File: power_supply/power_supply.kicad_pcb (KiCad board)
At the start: 2 copper layers, 100 x 100 mm, 36 parts, among them J1 Conn_01x02_Socket, J10 Conn_01x02_Socket, J11 Conn_01x02_Socket, J12 Conn_01x02_Socket, J13 Conn_01x02_Socket, J14 Conn_01x02_Socket, J15 Conn_01x02_Socket, J16 Conn_01x02_Socket, J17 Conn_01x02_Socket, J18 Conn_01x02_Socket, J19 Conn_01x02_Socket, J2 Conn_01x02_Socket, J20 Conn_01x02_Socket, J21 Conn_01x02_Pin, J22 Conn_01x02_Pin, J23 Conn_01x02_Socket, J24 Conn_01x02_Socket, J3 Conn_01x02_Socket, J4 Conn_01x02_Socket, J5 Conn_01x02_Socket, J6 Conn_01x02_Socket, J7 Conn_01x02_Socket, J8 Conn_01x02_Socket, J9 Conn_01x02_Socket

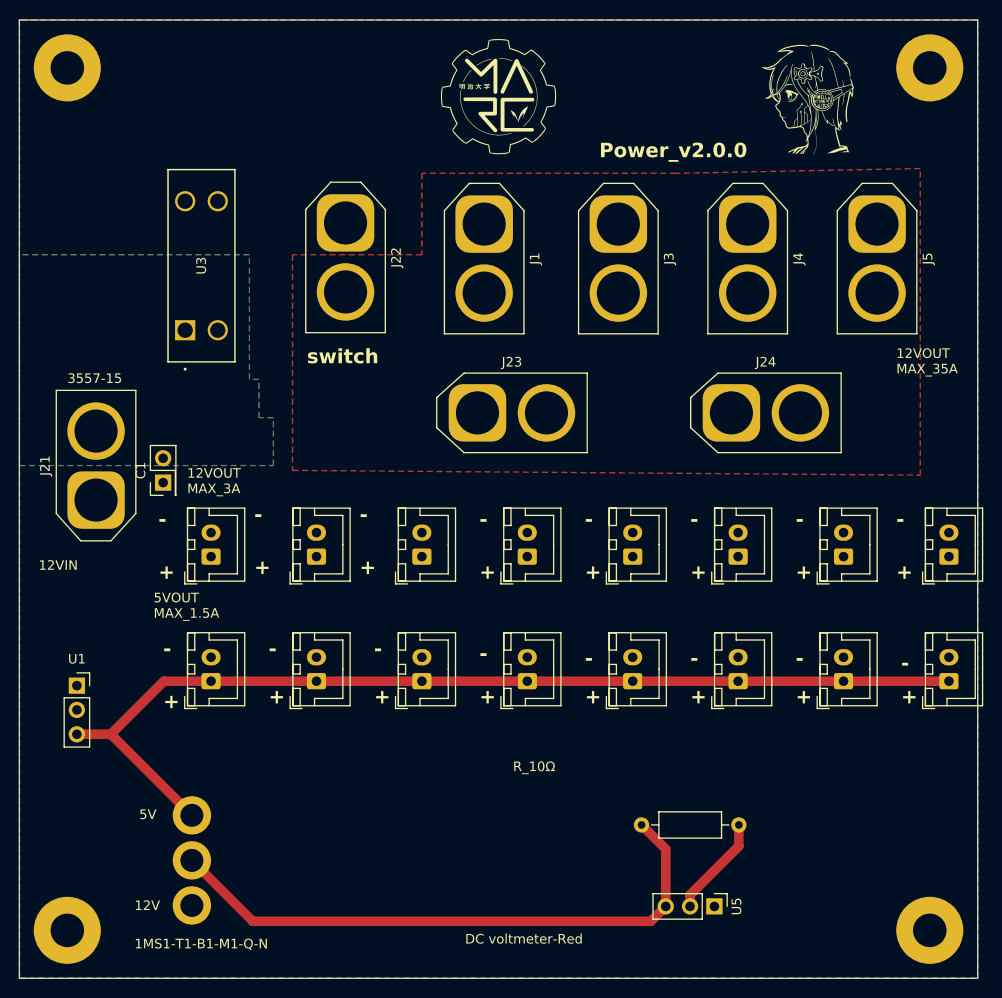
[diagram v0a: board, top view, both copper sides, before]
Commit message: 2024/11/08
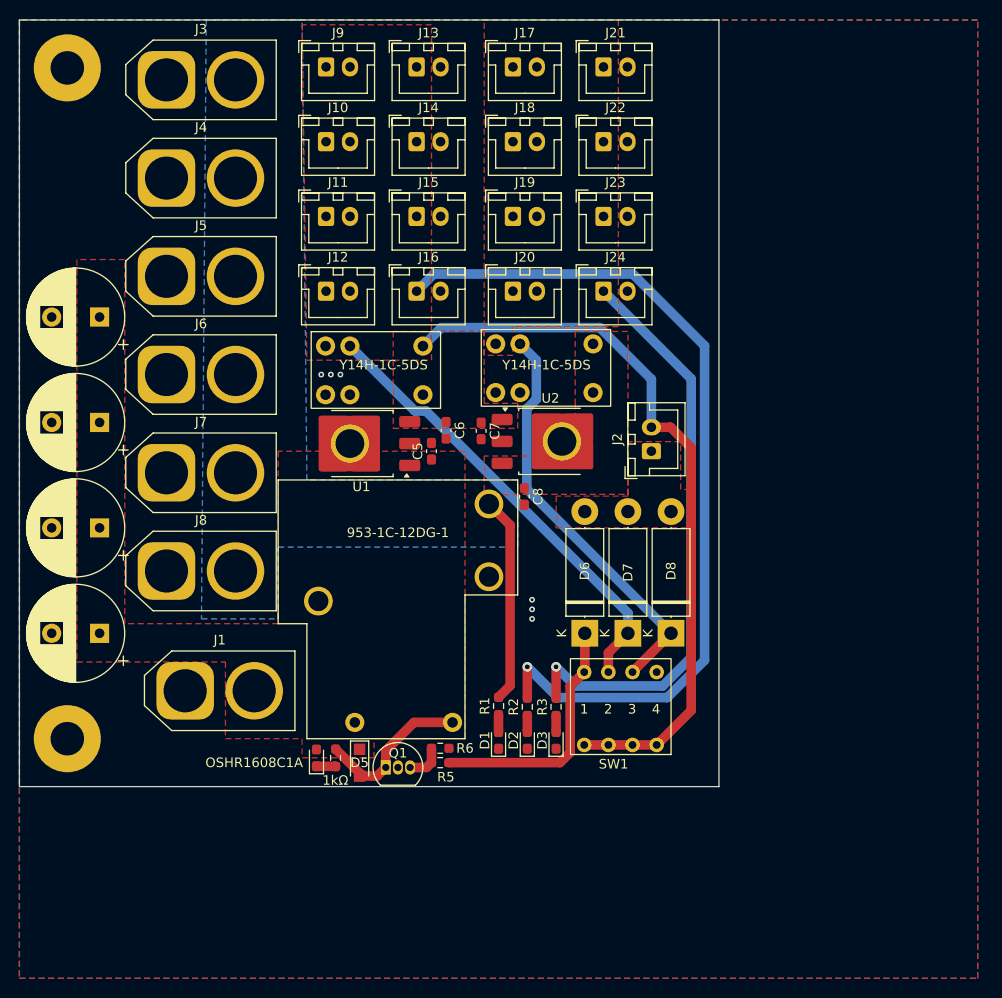
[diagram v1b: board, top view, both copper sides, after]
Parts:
- removed the G*** at (62.0, 20.0)
- removed the REF** at (107.0, 17.0)
- removed the REF** at (107.0, 107.0)
- added C2: C_Polarized, Capacitor_THT:CP_Radial_D10.0mm_P5.00mm, F.Cu at (20.4, 54.0)
- added C3: C_Polarized, Capacitor_THT:CP_Radial_D10.0mm_P5.00mm, F.Cu at (20.4, 65.0)
- added C4: C_Polarized, Capacitor_THT:CP_Radial_D10.0mm_P5.00mm, F.Cu at (20.4, 76.0)
- added C5: 0.33μF, Capacitor_SMD:C_0603_1608Metric_Pad1.08x0.95mm_HandSolder, F.Cu at (55.0, 57.0)
- added C6: 0.1μF, Capacitor_SMD:C_0603_1608Metric_Pad1.08x0.95mm_HandSolder, F.Cu at (56.5, 54.8)
- added C7: 0.33μF, Capacitor_SMD:C_0603_1608Metric_Pad1.08x0.95mm_HandSolder, F.Cu at (60.2, 54.9)
- added C8: 0.1μF, Capacitor_SMD:C_0603_1608Metric_Pad1.08x0.95mm_HandSolder, F.Cu at (64.7, 61.7)
- added D1: LED, LED_SMD:LED_0603_1608Metric_Pad1.05x0.95mm_HandSolder, F.Cu at (62.0, 87.2)
- added D2: LED, LED_SMD:LED_0603_1608Metric_Pad1.05x0.95mm_HandSolder, F.Cu at (65.0, 87.2)
- added D3: LED, LED_SMD:LED_0603_1608Metric_Pad1.05x0.95mm_HandSolder, F.Cu at (68.0, 87.2)
- added D4: OSHR1608C1A, LED_SMD:LED_0603_1608Metric_Pad1.05x0.95mm_HandSolder, F.Cu at (43.0, 89.0)
- added D5: GS1010FL, Diode_SMD:Nexperia_CFP3_SOD-123W, F.Cu at (47.5, 89.5)
- added D6: D, Diode_THT:D_5W_P12.70mm_Horizontal, F.Cu at (71.0, 76.0)
- added D7: D, Diode_THT:D_5W_P12.70mm_Horizontal, F.Cu at (75.5, 76.0)
- added D8: D, Diode_THT:D_5W_P12.70mm_Horizontal, F.Cu at (80.0, 76.0)
- added Q1: 2SC945L-K-T92-K, Package_TO_SOT_THT:TO-92_Inline, F.Cu at (50.2, 90.0)
- added R2: 300Ω, Resistor_SMD:R_0603_1608Metric_Pad0.98x0.95mm_HandSolder, F.Cu at (65.0, 83.7)
- added R3: 120Ω, Resistor_SMD:R_0603_1608Metric_Pad0.98x0.95mm_HandSolder, F.Cu at (68.0, 83.7)
- added R4: 1kΩ, Resistor_SMD:R_0603_1608Metric_Pad0.98x0.95mm_HandSolder, F.Cu at (45.0, 89.0)
- added R5: 1kΩ, Resistor_SMD:R_0603_1608Metric_Pad0.98x0.95mm_HandSolder, F.Cu at (55.9, 89.5)
- added R6: 10kΩ, Resistor_SMD:R_0603_1608Metric_Pad0.98x0.95mm_HandSolder, F.Cu at (55.9, 88.0)
- added SW1: SW_DIP_x04, 00a:KSD42, F.Cu at (78.5, 87.7)
- added U2: NJM2845DL1-33, 00a:TO-252-3_TabPin2, F.Cu at (67.4, 56.0)
- C1: value C -> C_Polarized; footprint Connector_PinHeader_2.54mm:PinHeader_2x01_P2.54mm_Vertical -> Capacitor_THT:CP_Radial_D10.0mm_P5.00mm
- G***: moved to B.Cu
- J1: value Conn_01x02_Socket -> XT60_IN
- J10, J11, J12, J13, J14, J15, J16, J9: value Conn_01x02_Socket -> XH_OUT
- J17, J18, J19, J20: value Conn_01x02_Socket -> XH_3.3V_OUT
- J2: value Conn_01x02_Socket -> Emergency Stop Switch
- J21, J22: value Conn_01x02_Pin -> XH_3.3V_OUT; footprint Connector_AMASS:AMASS_XT60-F_1x02_P7.20mm_Vertical -> Connector_JST:JST_XH_B2B-XH-A_1x02_P2.50mm_Vertical
- J23, J24: value Conn_01x02_Socket -> XH_3.3V_OUT; footprint Connector_AMASS:AMASS_XT60-F_1x02_P7.20mm_Vertical -> Connector_JST:JST_XH_B2B-XH-A_1x02_P2.50mm_Vertical
- J3, J4, J5: value Conn_01x02_Socket -> XT60_OUT
- J6, J7, J8: value Conn_01x02_Socket -> XT60_OUT; footprint Connector_JST:JST_XH_B2B-XH-A_1x02_P2.50mm_Vertical -> Connector_AMASS:AMASS_XT60-F_1x02_P7.20mm_Vertical
- R1: value 10 -> 1kΩ; footprint Resistor_THT:R_Axial_DIN0207_L6.3mm_D2.5mm_P10.16mm_Horizontal -> Resistor_SMD:R_0603_1608Metric_Pad0.98x0.95mm_HandSolder
- U1: value ~ -> NJM7805SDL1; footprint Connector_PinSocket_2.54mm:PinSocket_1x03_P2.54mm_Vertical -> 00a:TO-252-3_TabPin2
- U3: value ~ -> 953-1C-12DG-1; footprint footprints:3557-15_KEY -> 00a:953-1C-12DG-1
- U4: value ~ -> Y14H-1C-5DS; footprint 00a:1MS1-T1-B1-M1-Q-N-S -> 00a:Y14H-1C-5DS
- U5: value ~ -> Y14H-1C-5DS; footprint Connector_PinHeader_2.54mm:PinHeader_1x03_P2.54mm_Vertical -> 00a:Y14H-1C-5DS
- moved J13 75.5 mm to (53.5, 16.9), turned to 0 degrees
- moved J5 74.4 mm to (27.4, 38.8), turned to 0 degrees
- moved G*** 72.5 mm to (64.3, 85.7), turned to 180 degrees
- moved J21 69.6 mm to (73.0, 16.9), turned to 0 degrees
- moved J17 65.3 mm to (63.5, 16.9), turned to 0 degrees
- moved U5 63.0 mm to (61.7, 45.8), turned to 0 degrees
- moved J20 61.0 mm to (63.5, 40.3), turned to 0 degrees
- moved J18 61.0 mm to (63.5, 24.7), turned to 0 degrees
- moved J4 60.8 mm to (27.4, 28.5), turned to 0 degrees
- moved J12 60.7 mm to (44.0, 40.3), turned to 0 degrees
- moved J19 59.5 mm to (63.5, 32.5), turned to 0 degrees
- moved J1 57.8 mm to (29.3, 82.0), turned to 0 degrees
- moved J14 57.3 mm to (53.5, 24.7), turned to 0 degrees
- moved J11 55.8 mm to (44.0, 32.5), turned to 0 degrees
- moved J9 55.2 mm to (44.0, 16.9), turned to 0 degrees
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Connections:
- C1 pad 1: GND -> +12V_IN
- C1 pad 2: +12V_1 -> GND
- J1 pad 2: +12V_3 -> +12V_IN
- J10 pad 1: +12V_2 -> +5V_OUT
- J11 pad 1: +12V_2 -> +5V_OUT
- J12 pad 1: +12V_2 -> +5V_OUT
- J13 pad 1: +12V_2 -> +5V_OUT
- J14 pad 1: Net-(J14-Pin_1) -> +5V_OUT
- J15 pad 1: Net-(J14-Pin_1) -> +5V_OUT
- J16 pad 1: Net-(J14-Pin_1) -> +5V_OUT
- J17 pad 1: Net-(J14-Pin_1) -> +3.3V_OUT
- J18 pad 1: Net-(J14-Pin_1) -> +3.3V_OUT
- J19 pad 1: Net-(J14-Pin_1) -> +3.3V_OUT
- J2 pad 1: Net-(J14-Pin_1) -> Net-(D6-A)
- J2 pad 2: GND -> +5V_IN
- J20 pad 1: Net-(J14-Pin_1) -> +3.3V_OUT
- J21 pad 1: GND -> +3.3V_OUT
- J21 pad 2: +12V_1 -> GND
- J22 pad 1: +12V_2 -> +3.3V_OUT
- J22 pad 2: +12V_3 -> GND
- J23 pad 1: GND -> +3.3V_OUT
- J23 pad 2: +12V_3 -> GND
- J24 pad 1: GND -> +3.3V_OUT
- J24 pad 2: +12V_3 -> GND
- J3 pad 2: +12V_3 -> +12V_OUT
- J4 pad 2: +12V_3 -> +12V_OUT
- J5 pad 2: +12V_3 -> +12V_OUT
- J6 pad 1: +12V_2 -> GND
- J6 pad 2: GND -> +12V_OUT
- J7 pad 1: +12V_2 -> GND
- J7 pad 2: GND -> +12V_OUT
- J8 pad 1: +12V_2 -> GND
- J8 pad 2: GND -> +12V_OUT
- J9 pad 1: +12V_2 -> +5V_OUT
- R1 pad 1: Net-(R1-Pad1) -> Net-(D1-A)
- R1 pad 2: Net-(U5-OUT) -> +12V_OUT
- U1 pad 1: +12V_2 -> +12V_IN
- U1 pad 3: Net-(J14-Pin_1) -> +5V_IN
- U3 pad 1: +12V_1 -> +12V_IN
- U3 pad 2: +12V_1 -> Net-(D5-A)
- U3 pad 3: +12V_2 -> +12_IN
- U3 pad 4: +12V_2 -> unconnected-(U3-N.O.-Pad4)
- U4 pad 1: Net-(J14-Pin_1) -> +5V_OUT
- U4 pad 2: Net-(U5-OUT) -> unconnected-(U4-N.O.-Pad2)
- U4 pad 3: +12V_2 -> Net-(D7-K)
- U5 pad 1: GND -> +3.3V_OUT
- U5 pad 2: Net-(R1-Pad1) -> unconnected-(U5-N.O.-Pad2)
- U5 pad 3: Net-(U5-OUT) -> Net-(D8-K)
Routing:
- net Net-(J14-Pin_1): track 105.3 -> 0.00 mm
- net +5V_OUT: track 0.00 -> 91.4 mm, vias 0 -> 1
- net +5V_IN: track 0.00 -> 77.0 mm
- net Net-(U5-OUT): track 62.3 -> 0.00 mm
- net +3.3V_OUT: track 0.00 -> 61.4 mm, vias 0 -> 1
- net Net-(D7-K): track 0.00 -> 47.6 mm
- net Net-(D8-K): track 0.00 -> 43.3 mm
- net Net-(D6-K): track 0.00 -> 26.2 mm
- net +12V_OUT: track 0.00 -> 21.6 mm
- net Net-(D5-A): track 0.00 -> 16.9 mm
- net Net-(R1-Pad1): track 10.6 -> 0.00 mm
- net Net-(Q1-B): track 0.00 -> 3.94 mm
- net Net-(D4-K): track 0.00 -> 2.02 mm
- net Net-(D1-A): track 0.00 -> 1.80 mm
- net Net-(D3-A): track 0.00 -> 1.71 mm
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- added copper zone on F.Cu, net +12V_IN
- added copper zone on B.Cu, net +12V_OUT
- added copper zone on F.Cu, net +3.3V_IN
- added copper zone on F.Cu, net +3.3V_OUT
- added copper zone on F.Cu, net +5V_IN
- added copper zone on F.Cu, net +5V_OUT
- added copper zone on F.Cu, net GND
- added copper zone on F.Cu, net Net-(D6-A)
- removed copper zone on B.Cu, net +12V_1
- removed copper zone on F.Cu, net +12V_2
- removed copper zone on F.Cu, net +12V_3
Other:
- board size 100 x 100 mm -> 73 x 80 mm
- board text added: "https://github.com/syamei0/kicad/tree/master/power_supply"
- board text added: "power_supply_v3.0.0"
- board text added: "右下のスイッチで非常停止ボタンを 押した時に切る電源系統を 変更出来ます。 1:12V系統 2:5V系統 3:3.3V系統 4:無し"
- board text removed: "+"
- board text removed: "-"
- board text removed: "12V"
- board text removed: "12VIN"
- board text removed: "12VOUT MAX_35A"
- board text removed: "12VOUT MAX_3A"
- board text removed: "1MS1-T1-B1-M1-Q-N"
- board text removed: "3557-15"
- board text removed: "5V"
- board text removed: "5VOUT MAX_1.5A"
- board text removed: "DC voltmeter-Red"
- board text removed: "Power_v2.0.0"
- board text removed: "R_10Ω"
- board text removed: "switch"

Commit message: 2024/11/18
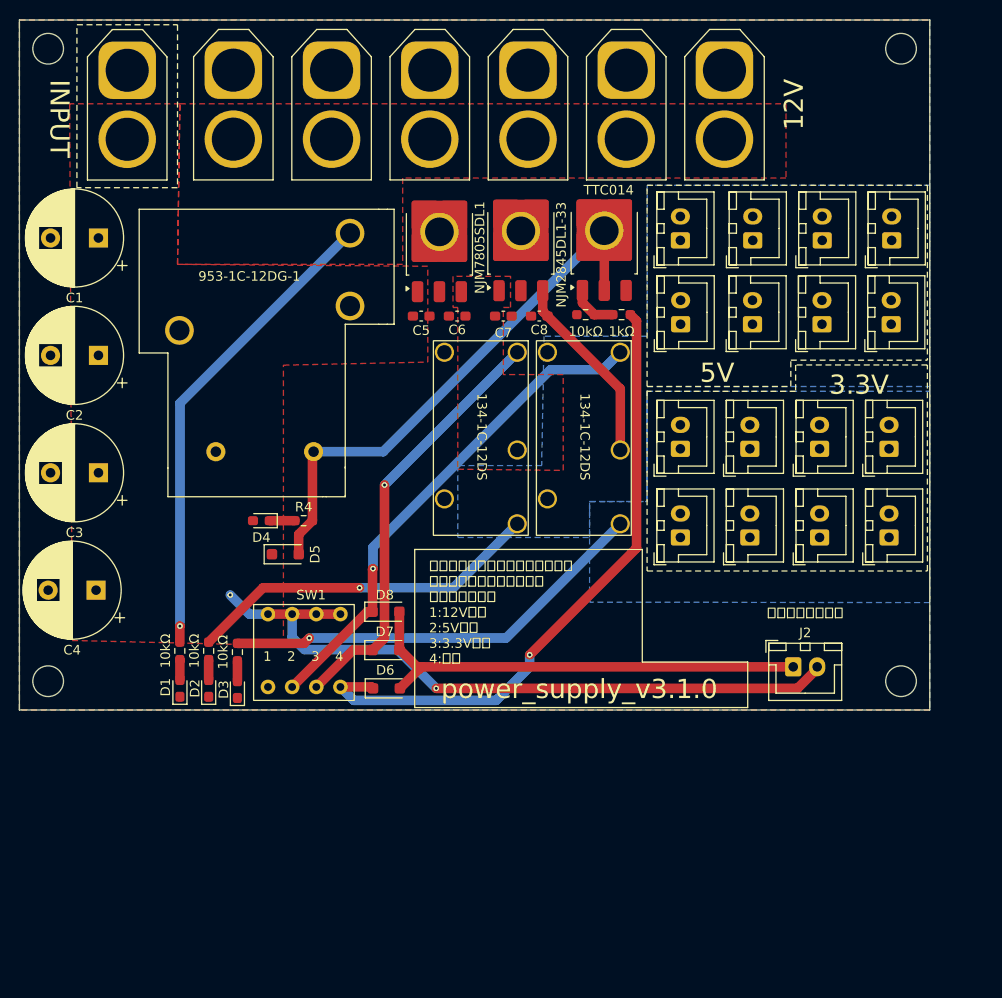
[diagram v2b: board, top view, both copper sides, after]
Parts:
- removed the REF** at (17.0, 17.0)
- removed the REF** at (17.0, 87.0)
- added G***: LOGO, 00a:MARC_rogo, B.Cu at (84.8, 73.5)
- added REF**: MountingHole_3.2mm_M3, MountingHole:MountingHole_3.2mm_M3, F.Cu at (104.0, 81.0)
- added REF**: MountingHole_3.2mm_M3, MountingHole:MountingHole_3.2mm_M3, F.Cu at (15.0, 81.0)
- added REF**: MountingHole_3.2mm_M3, MountingHole:MountingHole_3.2mm_M3, F.Cu at (104.0, 15.0)
- added REF**: MountingHole_3.2mm_M3, MountingHole:MountingHole_3.2mm_M3, F.Cu at (15.0, 15.0)
- D5: footprint Diode_SMD:Nexperia_CFP3_SOD-123W -> Diode_SMD:D_SOD-123F
- D6, D7, D8: footprint Diode_THT:D_5W_P12.70mm_Horizontal -> Diode_SMD:D_SOD-123F
- J1: footprint Connector_AMASS:AMASS_XT60-F_1x02_P7.20mm_Vertical -> Connector_AMASS:AMASS_XT60-M_1x02_P7.20mm_Vertical
- Q1: value 2SC945L-K-T92-K -> TTC014; footprint Package_TO_SOT_THT:TO-92_Inline -> 00a:TO-252-3_TabPin2
- R1, R4: value 1kΩ -> 10kΩ
- R2: value 300Ω -> 10kΩ
- R3: value 120Ω -> 10kΩ
- U4, U5: value Y14H-1C-5DS -> 134-1C-12DS; footprint 00a:Y14H-1C-5DS -> 00a:134-1C-12DS
- moved J1 65.0 mm to (23.2, 17.2), turned to -90 degrees
- moved Q1 59.4 mm to (73.0, 35.2), turned to 90 degrees
- moved J12 59.3 mm to (103.0, 35.0), turned to 90 degrees
- moved J3 58.2 mm to (85.6, 17.2), turned to -90 degrees
- moved J13 56.3 mm to (103.0, 43.8), turned to 90 degrees
- moved J11 53.0 mm to (95.8, 43.8), turned to 90 degrees
- moved J8 52.7 mm to (34.3, 17.2), turned to -90 degrees
- moved J17 52.1 mm to (81.0, 66.0), turned to 90 degrees
- moved R5 50.4 mm to (74.8, 42.8)
- moved J4 49.3 mm to (75.3, 17.2), turned to -90 degrees
- moved J10 48.4 mm to (88.5, 43.8), turned to 90 degrees
- moved J18 48.1 mm to (88.2, 66.0), turned to 90 degrees
- moved R6 47.7 mm to (71.1, 42.8), turned to 0 degrees
- moved J20 46.9 mm to (102.8, 66.0), turned to 90 degrees
- moved J19 46.3 mm to (95.5, 66.0), turned to 90 degrees
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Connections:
- J2 pad 2: +5V_IN -> +12V_IN
- Q1 pad 1: Net-(D5-A) -> Net-(Q1-B)
- Q1 pad 2: GND -> Net-(D5-A)
- Q1 pad 3: Net-(Q1-B) -> GND
- SW1 pad 1: +5V_IN -> +12V_IN
- SW1 pad 2: +5V_IN -> +12V_IN
- SW1 pad 3: +5V_IN -> +12V_IN
- SW1 pad 4: +5V_IN -> +12V_IN
- U3 pad 3: +12_IN -> +12V_IN
- U4 pad 1: +5V_OUT -> Net-(D7-K)
- U4 pad 2: unconnected-(U4-N.O.-Pad2) -> +5V_IN
- U4 pad 3: Net-(D7-K) -> +5V_OUT
- U4 pad 5: +5V_IN -> unconnected-(U4-Pad5)
- U5 pad 1: +3.3V_OUT -> Net-(D8-K)
- U5 pad 2: unconnected-(U5-N.O.-Pad2) -> +3.3V_IN
- U5 pad 3: Net-(D8-K) -> +3.3V_OUT
- U5 pad 5: +3.3V_IN -> unconnected-(U5-Pad5)
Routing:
- net +5V_IN: track 77.0 -> 0.00 mm
- net +12V_IN: track 0.00 -> 72.8 mm, vias 0 -> 2
- net +5V_OUT: track 91.4 -> 37.3 mm
- net Net-(D6-A): track 0.00 -> 48.9 mm
- net Net-(D6-K): track 26.2 -> 66.9 mm, vias 0 -> 1
- net Net-(D5-A): track 16.9 -> 57.5 mm
- net +12V_OUT: track 21.6 -> 50.0 mm, vias 0 -> 1
- net +3.3V_IN: track 0.00 -> 20.0 mm
- net +3.3V_OUT: track 61.4 -> 45.1 mm
- net Net-(D8-K): track 43.3 -> 52.6 mm, vias 0 -> 1
- net Net-(D7-K): track 47.6 -> 44.8 mm, vias 0 -> 1
- net Net-(Q1-B): track 3.94 -> 4.97 mm
- net Net-(D4-K): track 2.02 -> 2.62 mm
- net GND: vias 6 -> 0
- added copper zone on F.Cu, net +12V_OUT
- added copper zone on B.Cu, net +3.3V_OUT
- added copper zone on B.Cu, net +5V_OUT
- removed copper zone on B.Cu, net +12V_OUT
- removed copper zone on F.Cu, net +3.3V_IN
- removed copper zone on F.Cu, net +3.3V_OUT
- removed copper zone on F.Cu, net +5V_OUT
- removed copper zone on F.Cu, net Net-(D6-A)
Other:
- board size 73 x 80 mm -> 95 x 72 mm
- board text added: "12V"
- board text added: "3.3V"
- board text added: "5V"
- board text added: "D5,D6,D7,D8はダイオード D1,D2,D3,D4はLED"
- board text added: "INPUT"
- board text added: "https://partscabi.net/list/3c4d911b-a046-48f9-8f62-2c7ad6c0e181"
- board text added: "power_supply_v3.1.0"
- board text added: "左のスイッチで非常停止ボタンを 押した時に切る電源系統を 変更出来ます。 1:12V系統 2:5V系統 3:3.3V系統 4:無し"
- board text added: "非常停止スイッチ"
- board text removed: "power_supply_v3.0.0"
- board text removed: "右下のスイッチで非常停止ボタンを 押した時に切る電源系統を 変更出来ます。 1:12V系統 2:5V系統 3:3.3V系統 4:無し"
